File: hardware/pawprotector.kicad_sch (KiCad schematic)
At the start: 19 parts, among them J1 USB_A, J2 USB_A, U1 TPS2514A, U2 TPD2E001, U3 TPS2561

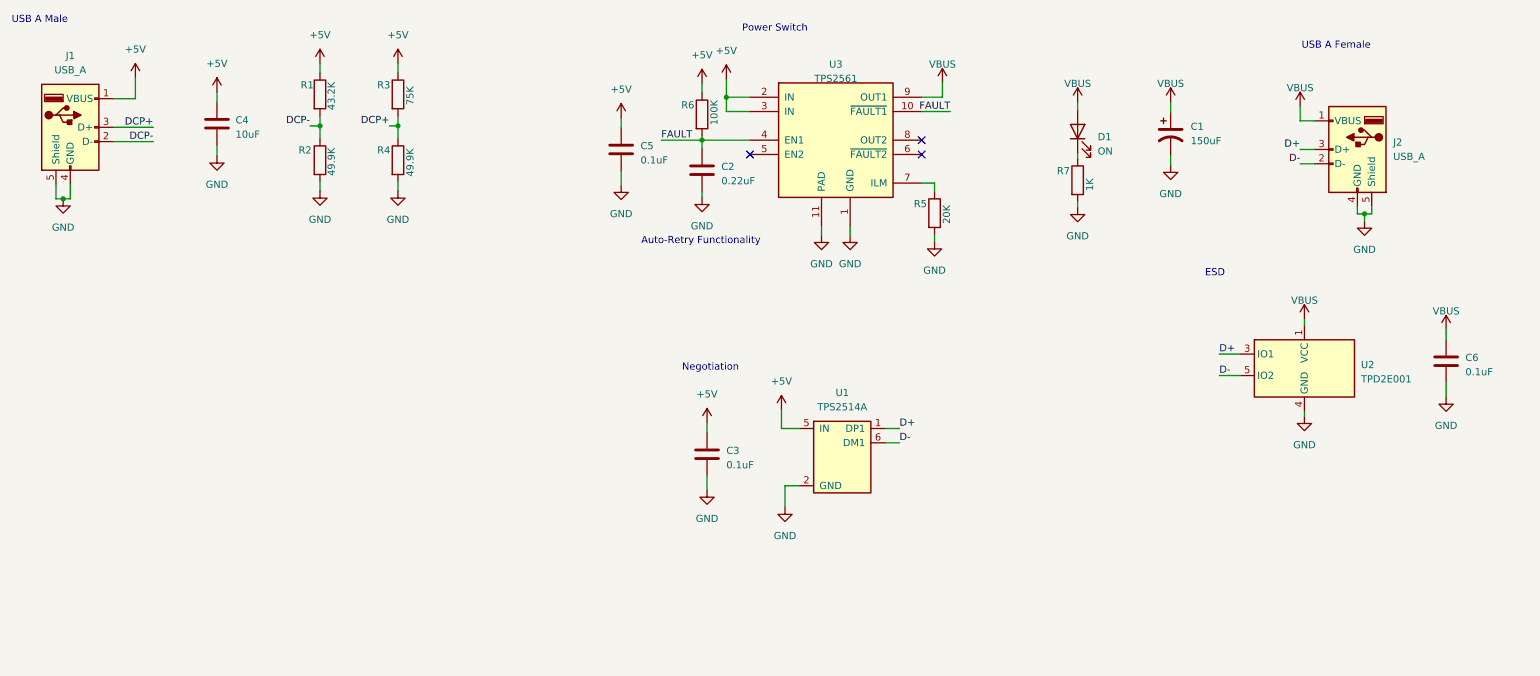
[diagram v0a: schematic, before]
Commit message: Usb-c
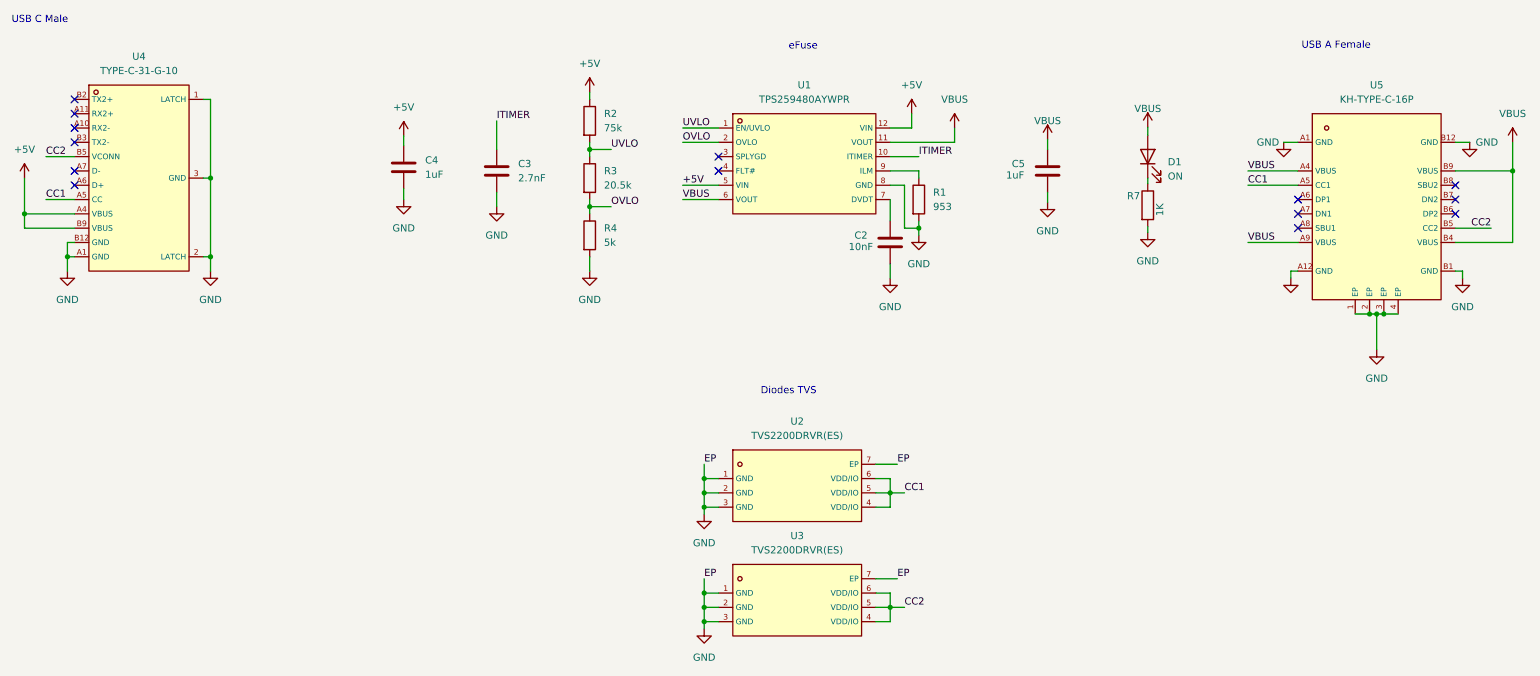
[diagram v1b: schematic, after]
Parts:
- removed C1: 150uF, Capacitor_SMD:CP_Elec_6.3x5.4, symbol Device:C_Polarized_US
- removed C6: 0.1uF, Capacitor_SMD:C_0402_1005Metric, symbol Device:C
- removed J1: USB_A, usbCondom:C46394, symbol Connector:USB_A
- removed J2: USB_A, usbCondom:875832010BLF, symbol Connector:USB_A
- removed R5: 20K, Resistor_SMD:R_0402_1005Metric, symbol Device:R
- removed R6: 100K, Resistor_SMD:R_0402_1005Metric, symbol Device:R
- removed U1: TPS2514A, Package_TO_SOT_SMD:SOT-23-6, symbol Interface_USB:TPS2514A
- removed U2: TPD2E001, Package_TO_SOT_SMD:SOT-553, symbol usbCondom:TPD2E001DRLR
- removed U3: TPS2561, Package_SON:VSON-10-1EP_3x3mm_P0.5mm_EP1.65x2.4mm_ThermalVias, symbol Interface_USB:TPS2561
- added U1: TPS259480AYWPR, TPS259480:POWERWCSP-12_L2.5-W1.7_TPS259482AYWPR, symbol TPS259480AYWPR2.0:TPS259480AYWPR
- added U2, U3: TVS2200DRVR(ES), TVS2200:DFN-6_L2.0-W2.0-P0.65-BL-EP1.6, symbol TVS2200DRVR(ES):TVS2200DRVR(ES)
- added U4: TYPE-C-31-G-10, USB-C_Male:USB-C-SMD_TYPE-C-31-G-10, symbol TYPE-C-31-G-10:TYPE-C-31-G-10
- added U5: KH-TYPE-C-16P, USB-C-FEMALE:USB-C-SMD_KH-TYPE-C-16P, symbol KH-TYPE-C-16P:KH-TYPE-C-16P
- C2: value 0.22uF -> 10nF; footprint Capacitor_SMD:C_0402_1005Metric -> Capacitor_SMD:C_0603_1608Metric; LCSC# C16772 -> C100042
- C3: value 0.1uF -> 2.7nF; LCSC# C392963 -> C106251
- C4: value 10uF -> 1uF; footprint Capacitor_SMD:C_0805_2012Metric -> Capacitor_SMD:C_0603_1608Metric; LCSC# C3015160 -> C5199872
- C5: value 0.1uF -> 1uF; footprint Capacitor_SMD:C_0402_1005Metric -> Capacitor_SMD:C_0603_1608Metric; LCSC# C392963 -> C5199872
- R1: value 43.2K -> 953; LCSC# C2906870 -> C42372098
- R2: value 49.9K -> 75k; footprint Resistor_SMD:R_0402_1005Metric -> Resistor_SMD:R_0603_1608Metric; LCSC# C2906873 -> C2907067
- R3: value 75K -> 20.5k; footprint Resistor_SMD:R_0402_1005Metric -> Resistor_SMD:R_0603_1608Metric; LCSC# C328330 -> C203395
- R4: value 49.9K -> 5k; footprint Resistor_SMD:R_0402_1005Metric -> Resistor_SMD:R_0603_1608Metric; LCSC# C2906873 -> C166926
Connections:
- net +5V: now also R2.1, U1.12 (VIN), U1.5 (VIN), U4.A4 (VBUS), U4.B9 (VBUS); no longer C3.1, C5.1, R1.1, R3.1
- net GND: now also R1.2, U1.8 (GND), U2.1 (GND), U2.2 (GND), U2.3 (GND), U2.7 (EP), U3.1 (GND), U3.2 (GND), U3.3 (GND), U3.7 (EP), U4.1 (LATCH), U4.2 (LATCH), U4.3 (GND), U4.A1 (GND), U4.B12 (GND), U5.1 (EP), U5.2 (EP), U5.3 (EP), U5.4 (EP), U5.A1 (GND), U5.A12 (GND), U5.B1 (GND), U5.B12 (GND); no longer R2.2
- net VBUS: now also C5.1, U1.11 (VOUT), U1.6 (VOUT), U5.A4 (VBUS), U5.A9 (VBUS), U5.B4 (VBUS), U5.B9 (VBUS)
- net DCP+ renamed OVLO
- net OVLO: now also U1.2 (OVLO)
- removed net DCP-: R1.2, R2.1
- net FAULT: no longer names the net of C2.1
- net FAULT: now also U1.7 (DVDT)
- new net: R1.1, U1.9 (ILM)
- new net CC1: U2.4 (VDD/IO), U2.5 (VDD/IO), U2.6 (VDD/IO), U4.A5 (CC), U5.A5 (CC1)
- new net CC2: U3.4 (VDD/IO), U3.5 (VDD/IO), U3.6 (VDD/IO), U4.B5 (VCONN), U5.B5 (CC2)
- new net ITIMER: C3.1, U1.10 (ITIMER)
- new net UVLO: R2.2, R3.1, U1.1 (EN/UVLO)
- no-connect marks 3 -> 14
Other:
- note added: "Diodes TVS"
- note added: "USB C Male"
- note added: "eFuse"
- note removed: "Auto-Retry Functionality"
- note removed: "ESD"
- note removed: "Negotiation"
- note removed: "Power Switch"
- note removed: "USB A Male"
- moved on the sheet: C4, D1, R7
